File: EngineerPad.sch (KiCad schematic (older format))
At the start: 69 parts, among them J1 AVR ISP, J2 USB_A, SW1 SW_Push, SW10 SW_Push, SW11 SW_Push, SW12 SW_Push, SW13 SW_Push, SW14 SW_Push, SW15 SW_Push, SW16 SW_Push, SW17 SW_Push, SW18 SW_Push, SW19 SW_Push, SW2 SW_Push, SW20 SW_Push, SW21 SW_Push, SW22 SW_Push, SW23 SW_Push, SW3 SW_Push, SW4 SW_Push, SW5 SW_Push, SW6 SW_Push, SW7 SW_Push, SW8 SW_Push, SW9 SW_Push, U1 ATmega328P-PU, Y1 16MHz

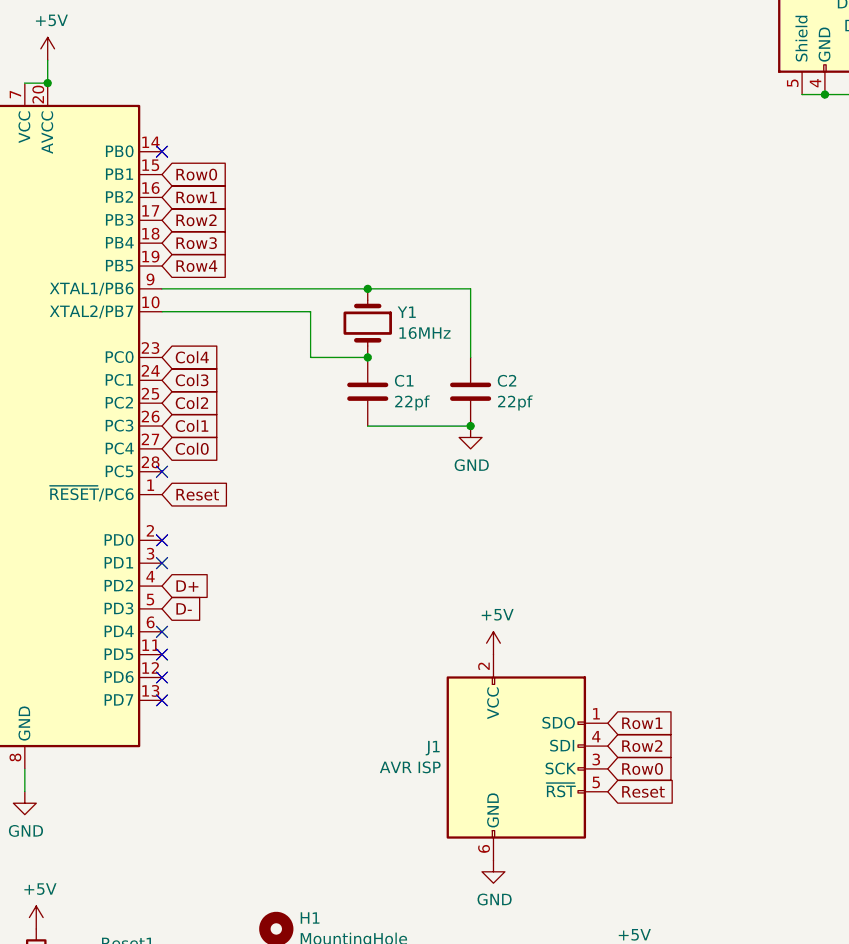
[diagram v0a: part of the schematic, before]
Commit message: wip
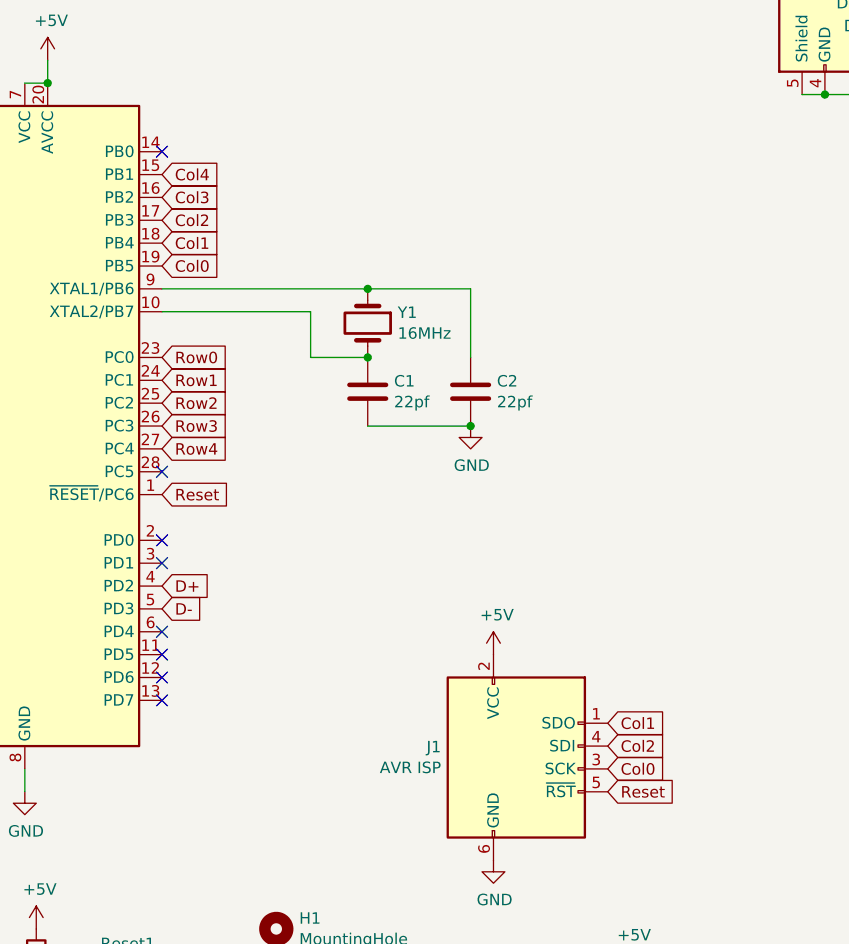
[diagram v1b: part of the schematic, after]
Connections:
- net Col0: now also J1.3 (SCK), U1.19 (PB5); no longer U1.27 (PC4)
- net Col1: now also J1.1 (SDO), U1.18 (PB4); no longer U1.26 (PC3)
- net Col2: now also J1.4 (SDI), U1.17 (PB3); no longer U1.25 (PC2)
- net Col3: now also U1.16 (PB2); no longer U1.24 (PC1)
- net Col4: now also U1.15 (PB1); no longer U1.23 (PC0)
- net Row0: now also U1.23 (PC0); no longer J1.3 (SCK), U1.15 (PB1)
- net Row1: now also U1.24 (PC1); no longer J1.1 (SDO), U1.16 (PB2)
- net Row2: now also U1.25 (PC2); no longer J1.4 (SDI), U1.17 (PB3)
- net Row3: now also U1.26 (PC3); no longer U1.18 (PB4)
- net Row4: now also U1.27 (PC4); no longer U1.19 (PB5)
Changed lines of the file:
@@
 Reset
 Text GLabel 4400 5200 2    50   Input ~ 0
-Row0
+Col0
 Text GLabel 4400 5100 2    50   Input ~ 0
-Row2
-Text GLabel 2450 2900 2    50   Input ~ 0
+Col2
+Text GLabel 2450 3700 2    50   Input ~ 0
 Row3
-Text GLabel 2450 2800 2    50   Input ~ 0
+Text GLabel 2450 3600 2    50   Input ~ 0
 Row2
 $Comp
@@
 Col0
 Connection ~ 8850 1350
-Text GLabel 2450 2600 2    50   Input ~ 0
+Text GLabel 2450 3400 2    50   Input ~ 0
 Row0
-Text GLabel 2450 2700 2    50   Input ~ 0
+Text GLabel 2450 3500 2    50   Input ~ 0
 Row1
-Text GLabel 2450 3800 2    50   Input ~ 0
+Text GLabel 2450 3000 2    50   Input ~ 0
 Col0
-Text GLabel 2450 3700 2    50   Input ~ 0
+Text GLabel 2450 2900 2    50   Input ~ 0
 Col1
 NoConn ~ 2450 2500
@@
 Text GLabel 10350 850  1    50   Input ~ 0
 Col4
-Text GLabel 2450 3000 2    50   Input ~ 0
+Text GLabel 2450 3800 2    50   Input ~ 0
 Row4
-Text GLabel 2450 3600 2    50   Input ~ 0
+Text GLabel 2450 2800 2    50   Input ~ 0
 Col2
-Text GLabel 2450 3500 2    50   Input ~ 0
+Text GLabel 2450 2700 2    50   Input ~ 0
 Col3
-Text GLabel 2450 3400 2    50   Input ~ 0
+Text GLabel 2450 2600 2    50   Input ~ 0
 Col4
 Connection ~ 8350 1350
@@
 NoConn ~ 9150 5350
 Text GLabel 4400 5000 2    50   Input ~ 0
-Row1
+Col1
 NoConn ~ 2450 4200
 NoConn ~ 2450 4300

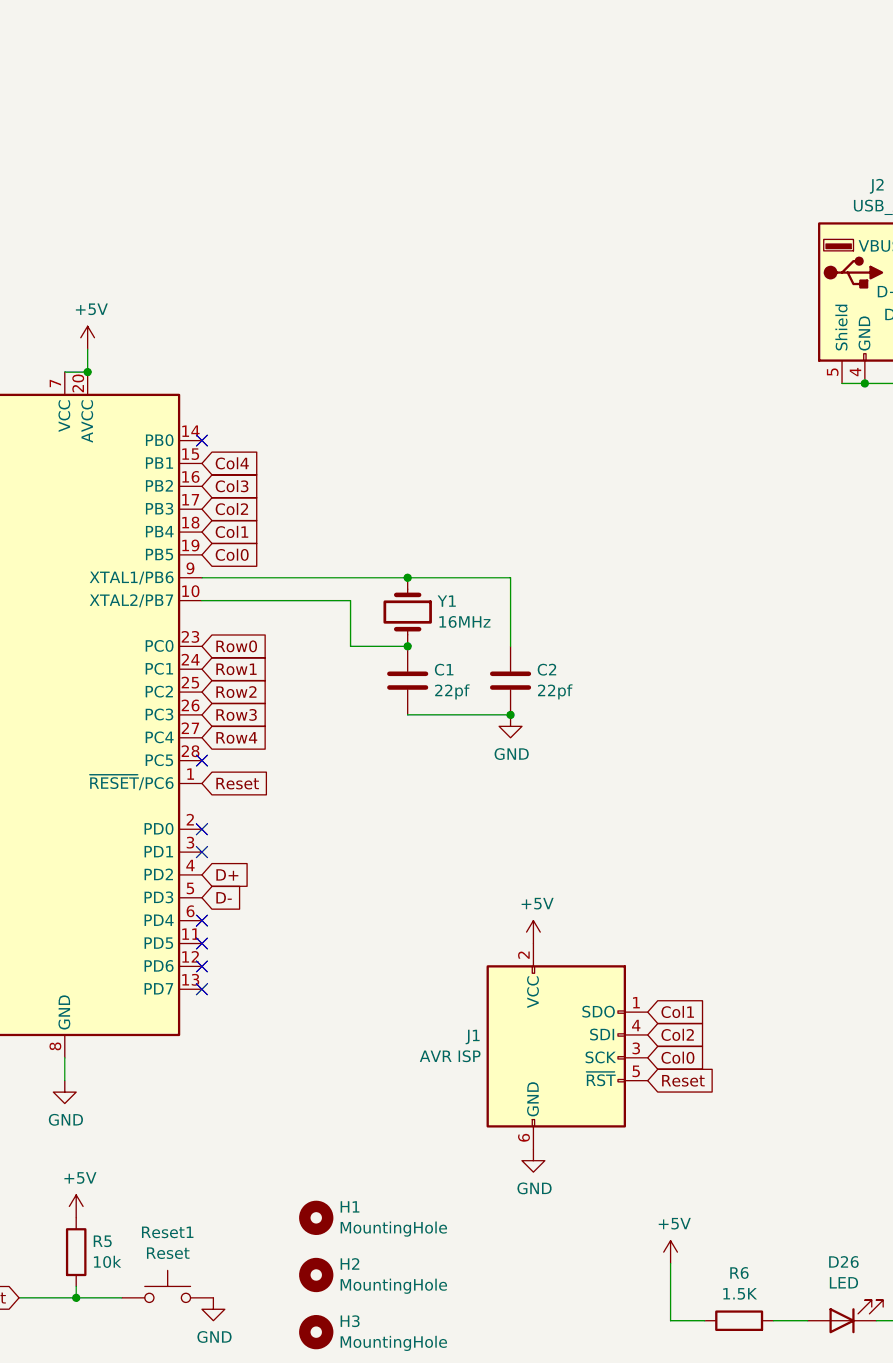
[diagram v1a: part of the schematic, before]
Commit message: handwired
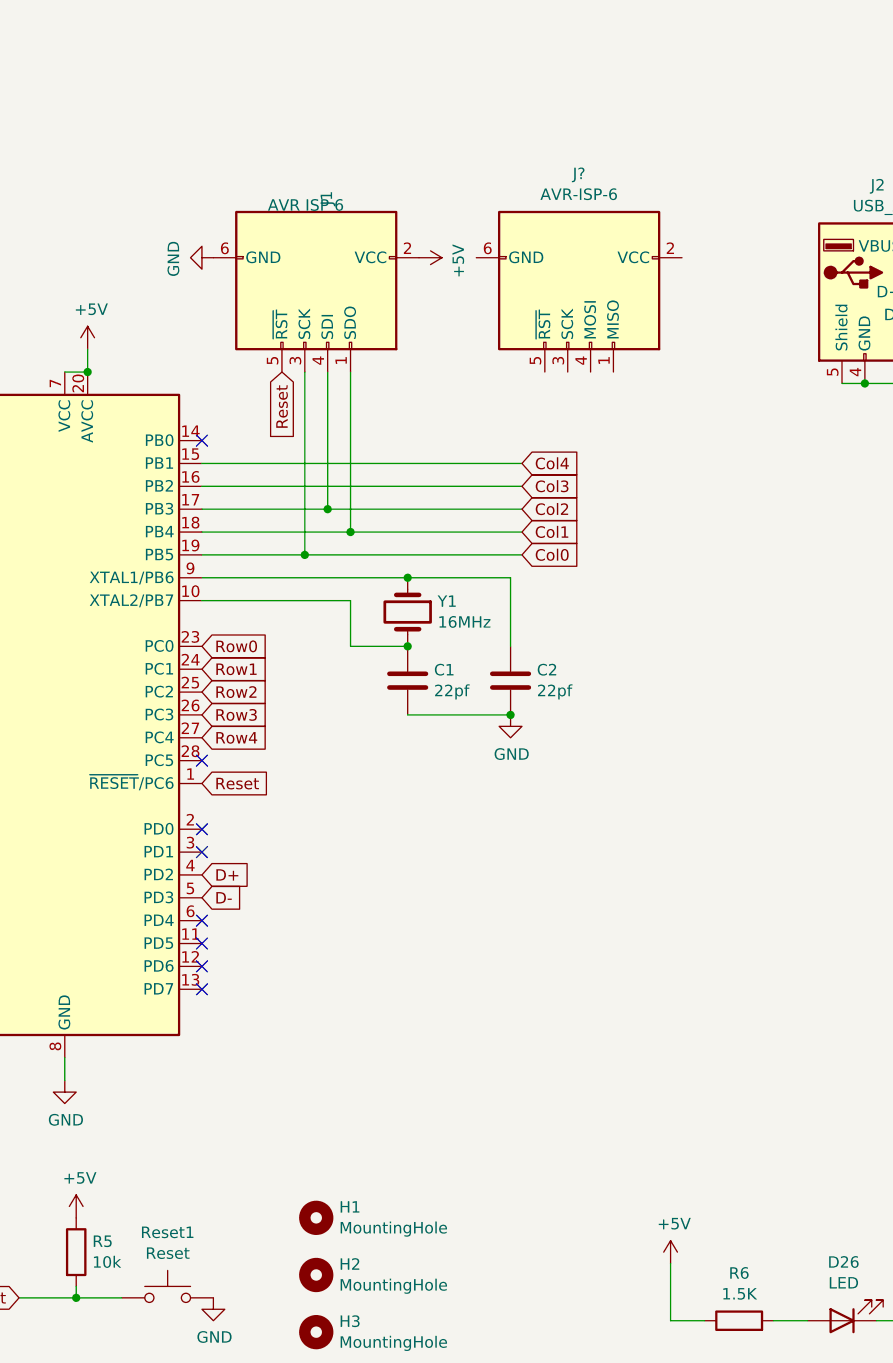
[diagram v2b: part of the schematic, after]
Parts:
- added J?: AVR-ISP-6, symbol Connector:AVR-ISP-6
- J1: value AVR ISP -> AVR ISP 6
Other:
- moved on the sheet: J1
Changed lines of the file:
@@
 L power:+5V #PWR04
 U 1 1 5F169608
-P 3900 4700
-F 0 "#PWR04" H 3900 4550 50  0001 C CNN
-F 1 "+5V" H 3915 4873 50  0000 C CNN
-F 2 "" H 3900 4700 50  0001 C CNN
-F 3 "" H 3900 4700 50  0001 C CNN
-	1    3900 4700
-	1    0    0    -1
+P 3400 1700
+F 0 "#PWR04" H 3400 1550 50  0001 C CNN
+F 1 "+5V" H 3415 1873 50  0000 C CNN
+F 2 "" H 3400 1700 50  0001 C CNN
+F 3 "" H 3400 1700 50  0001 C CNN
+	1    3400 1700
+	0    1    1    0
 $EndComp
 $Comp
 L power:GND #PWR07
 U 1 1 5F169EF0
-P 3900 5600
-F 0 "#PWR07" H 3900 5350 50  0001 C CNN
-F 1 "GND" H 3905 5427 50  0000 C CNN
-F 2 "" H 3900 5600 50  0001 C CNN
-F 3 "" H 3900 5600 50  0001 C CNN
-	1    3900 5600
-	1    0    0    -1
+P 2500 1700
+F 0 "#PWR07" H 2500 1450 50  0001 C CNN
+F 1 "GND" H 2505 1527 50  0000 C CNN
+F 2 "" H 2500 1700 50  0001 C CNN
+F 3 "" H 2500 1700 50  0001 C CNN
+	1    2500 1700
+	0    1    1    0
 $EndComp
 $Comp
@@
 	1    0    0    -1
 $EndComp
-Text GLabel 4400 5300 2    50   Input ~ 0
+Text GLabel 2800 2200 3    50   Input ~ 0
 Reset
-Text GLabel 4400 5200 2    50   Input ~ 0
-Col0
-Text GLabel 4400 5100 2    50   Input ~ 0
-Col2
 Text GLabel 2450 3700 2    50   Input ~ 0
 Row3
@@
 Text GLabel 2450 3500 2    50   Input ~ 0
 Row1
-Text GLabel 2450 3000 2    50   Input ~ 0
+Text GLabel 3850 3000 2    50   Input ~ 0
 Col0
-Text GLabel 2450 2900 2    50   Input ~ 0
+Text GLabel 3850 2900 2    50   Input ~ 0
 Col1
 NoConn ~ 2450 2500
@@
 Text GLabel 2450 3800 2    50   Input ~ 0
 Row4
-Text GLabel 2450 2800 2    50   Input ~ 0
+Text GLabel 3850 2800 2    50   Input ~ 0
 Col2
-Text GLabel 2450 2700 2    50   Input ~ 0
+Text GLabel 3850 2700 2    50   Input ~ 0
 Col3
-Text GLabel 2450 2600 2    50   Input ~ 0
+Text GLabel 3850 2600 2    50   Input ~ 0
 Col4
 Connection ~ 8350 1350
@@
 NoConn ~ 2450 4900
 NoConn ~ 9150 5350
-Text GLabel 4400 5000 2    50   Input ~ 0
-Col1
 NoConn ~ 2450 4200
 NoConn ~ 2450 4300
@@
 L JSA:Oshwa_ISP_6 J1
 U 1 1 5F1679A9
-P 4000 5200
-F 0 "J1" H 3671 5296 50  0000 R CNN
-F 1 "AVR ISP" H 3671 5205 50  0000 R CNN
-F 2 "JSA:AVRISP" V 3750 5250 50  0001 C CNN
-F 3 "https://www.oshwa.org/a-resolution-to-redefine-spi-signal-names" H 2725 4650 50  0001 C CNN
-	1    4000 5200
-	1    0    0    -1
+P 2900 1800
+F 0 "J1" H 2571 1896 50  0000 R CNN
+F 1 "AVR ISP 6" V 2571 1805 50  0000 C CNN
+F 2 "JSA:AVRISP" V 2650 1850 50  0001 C CNN
+F 3 "https://www.oshwa.org/a-resolution-to-redefine-spi-signal-names" H 1625 1250 50  0001 C CNN
+	1    2900 1800
+	0    1    1    0
 $EndComp
 $Comp
@@
 	1    0    0    -1
 $EndComp
+Wire Wire Line
+	2900 2200 2900 3000
+Wire Wire Line
+	2900 3000 2450 3000
+Wire Wire Line
+	3000 2200 3000 2800
+Wire Wire Line
+	3000 2800 2450 2800
+Wire Wire Line
+	3100 2200 3100 2900
+Wire Wire Line
+	3100 2900 2450 2900
+Wire Wire Line
+	2900 3000 3850 3000
+Connection ~ 2900 3000
+Wire Wire Line
+	3100 2900 3850 2900
+Connection ~ 3100 2900
+Wire Wire Line
+	3000 2800 3850 2800
+Connection ~ 3000 2800
+Wire Wire Line
+	2450 2700 3850 2700
+Wire Wire Line
+	2450 2600 3850 2600
+$Comp
+L Connector:AVR-ISP-6 J?
+U 1 1 5F4E2942
+P 4050 1800
+F 0 "J?" V 3583 1850 50  0000 C CNN
+F 1 "AVR-ISP-6" V 3674 1850 50  0000 C CNN
+F 2 "" V 3800 1850 50  0001 C CNN
+F 3 " ~" H 2775 1250 50  0001 C CNN
+	1    4050 1800
+	0    1    1    0
+$EndComp
 $EndSCHEMATC
